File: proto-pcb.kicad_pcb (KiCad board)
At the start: 2 copper layers, 48 x 100 mm, 624 parts

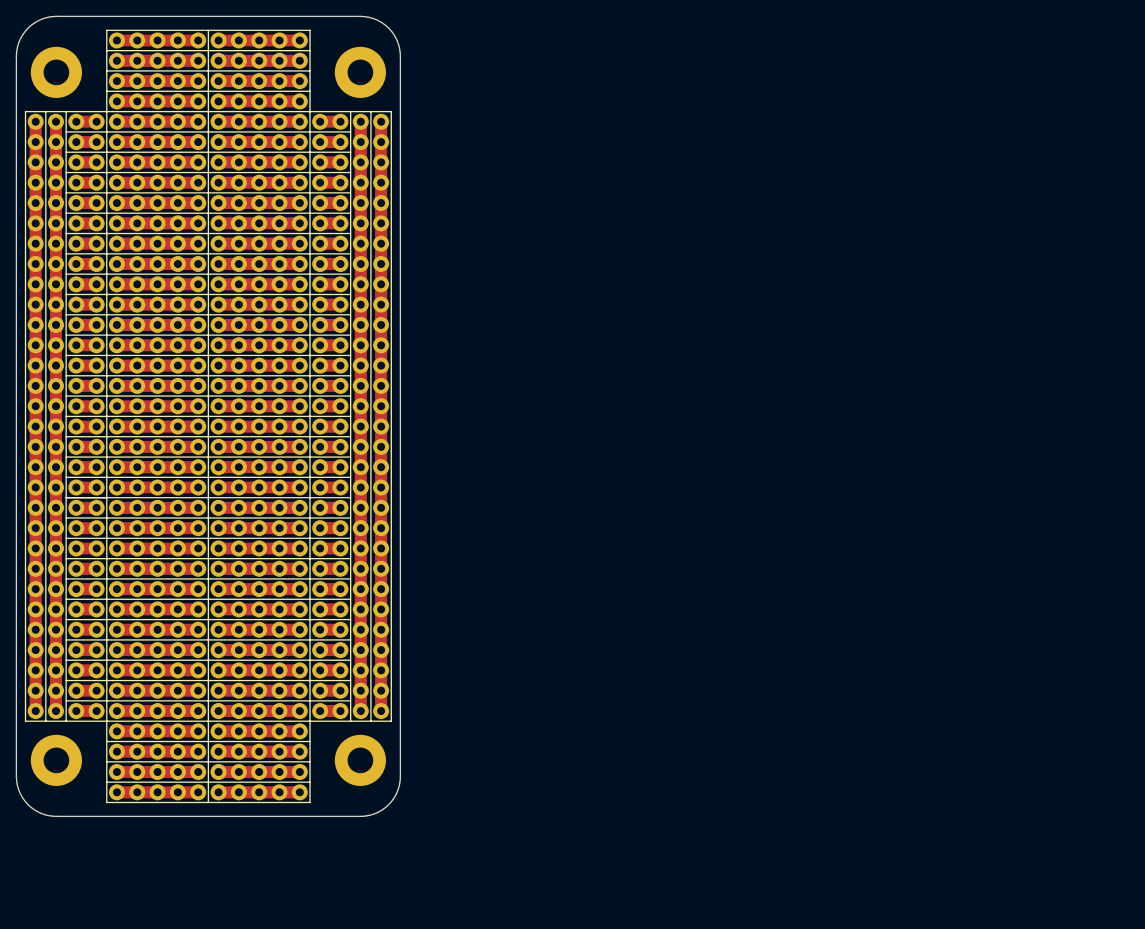
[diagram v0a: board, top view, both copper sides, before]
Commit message: KiCAD
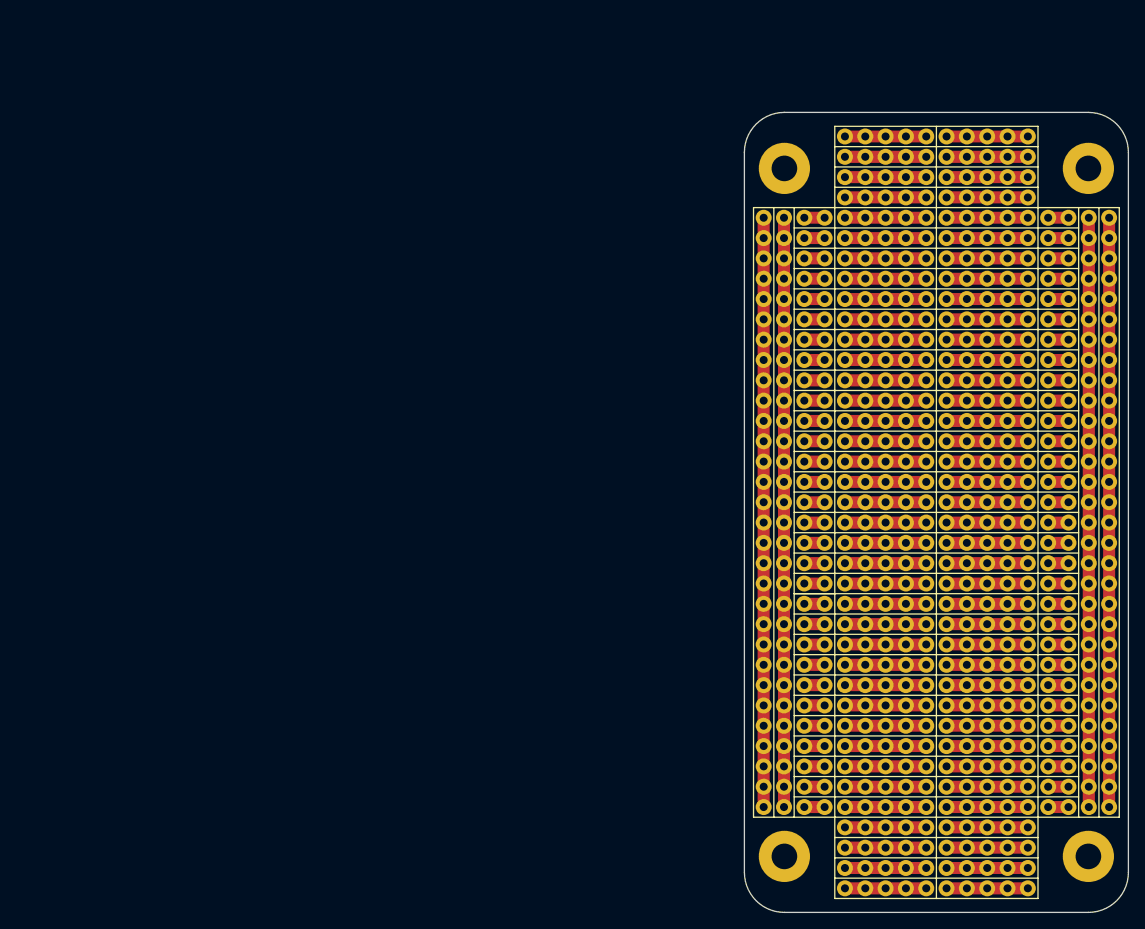
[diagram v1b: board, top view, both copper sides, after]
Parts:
- moved REF** 91.8 mm to (156.2, 100.3)
- moved REF** 91.8 mm to (146.1, 102.9)
- moved REF** 91.8 mm to (156.2, 67.3)
- moved REF** 91.8 mm to (156.2, 102.9)
- moved REF** 91.8 mm to (146.1, 143.5)
- moved REF** 91.8 mm to (156.2, 125.7)
- moved REF** 91.8 mm to (146.1, 57.1)
- moved REF** 91.8 mm to (146.1, 115.6)
- moved REF** 91.8 mm to (146.1, 133.3)
- moved REF** 91.8 mm to (146.1, 105.4)
- moved REF** 91.8 mm to (156.2, 95.2)
- moved REF** 91.8 mm to (156.2, 80.0)
- moved REF** 91.8 mm to (146.1, 118.1)
- moved REF** 91.8 mm to (156.2, 113.0)
- moved REF** 91.8 mm to (146.1, 113.0)
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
